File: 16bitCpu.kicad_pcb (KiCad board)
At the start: 4 copper layers, 73 parts, among them SW1 SW_Push, SW2 SW_SPDT, U1 74LS245, U10 74LS86, U11 74LS245, U12 74LS173, U13 74LS173, U14 74LS245, U15 74LS173, U16 74LS173, U17 74LS245, U18 74LS173, U19 74LS173, U2 74LS245, U20 74LS245, U21 74LS173, U22 74LS173, U23 LM555xN, U24 74LS04, U25 74LS08, U26 74LS32, U27 LM555xN, U28 LM555xN, U29 74LS245, U3 74LS283, U30 74LS245, U31 74LS161, U32 74LS161, U33 74LS161, U34 74LS161, U35 74HC00, U36 74LS245, U37 74HC04, U38 74LS173, U39 74LS173, U4 74LS283, U40 74LS245, U41 74LS173, U42 74LS173, U43 AS6C6264, U44 AS6C6264, U45 AT28C64B-15PU, U46 AT28C64B-15PU, U47 74LS245, U48 74LS173, U49 74LS173, U5 74LS283, U50 74LS245, U51 74LS173, U52 74LS173, U53 74LS173, U54 74HC02, U55 74HC02, U56 74LS08, U57 74LS08, U6 74LS283, U7 74LS86, U8 74LS86, U9 74LS86

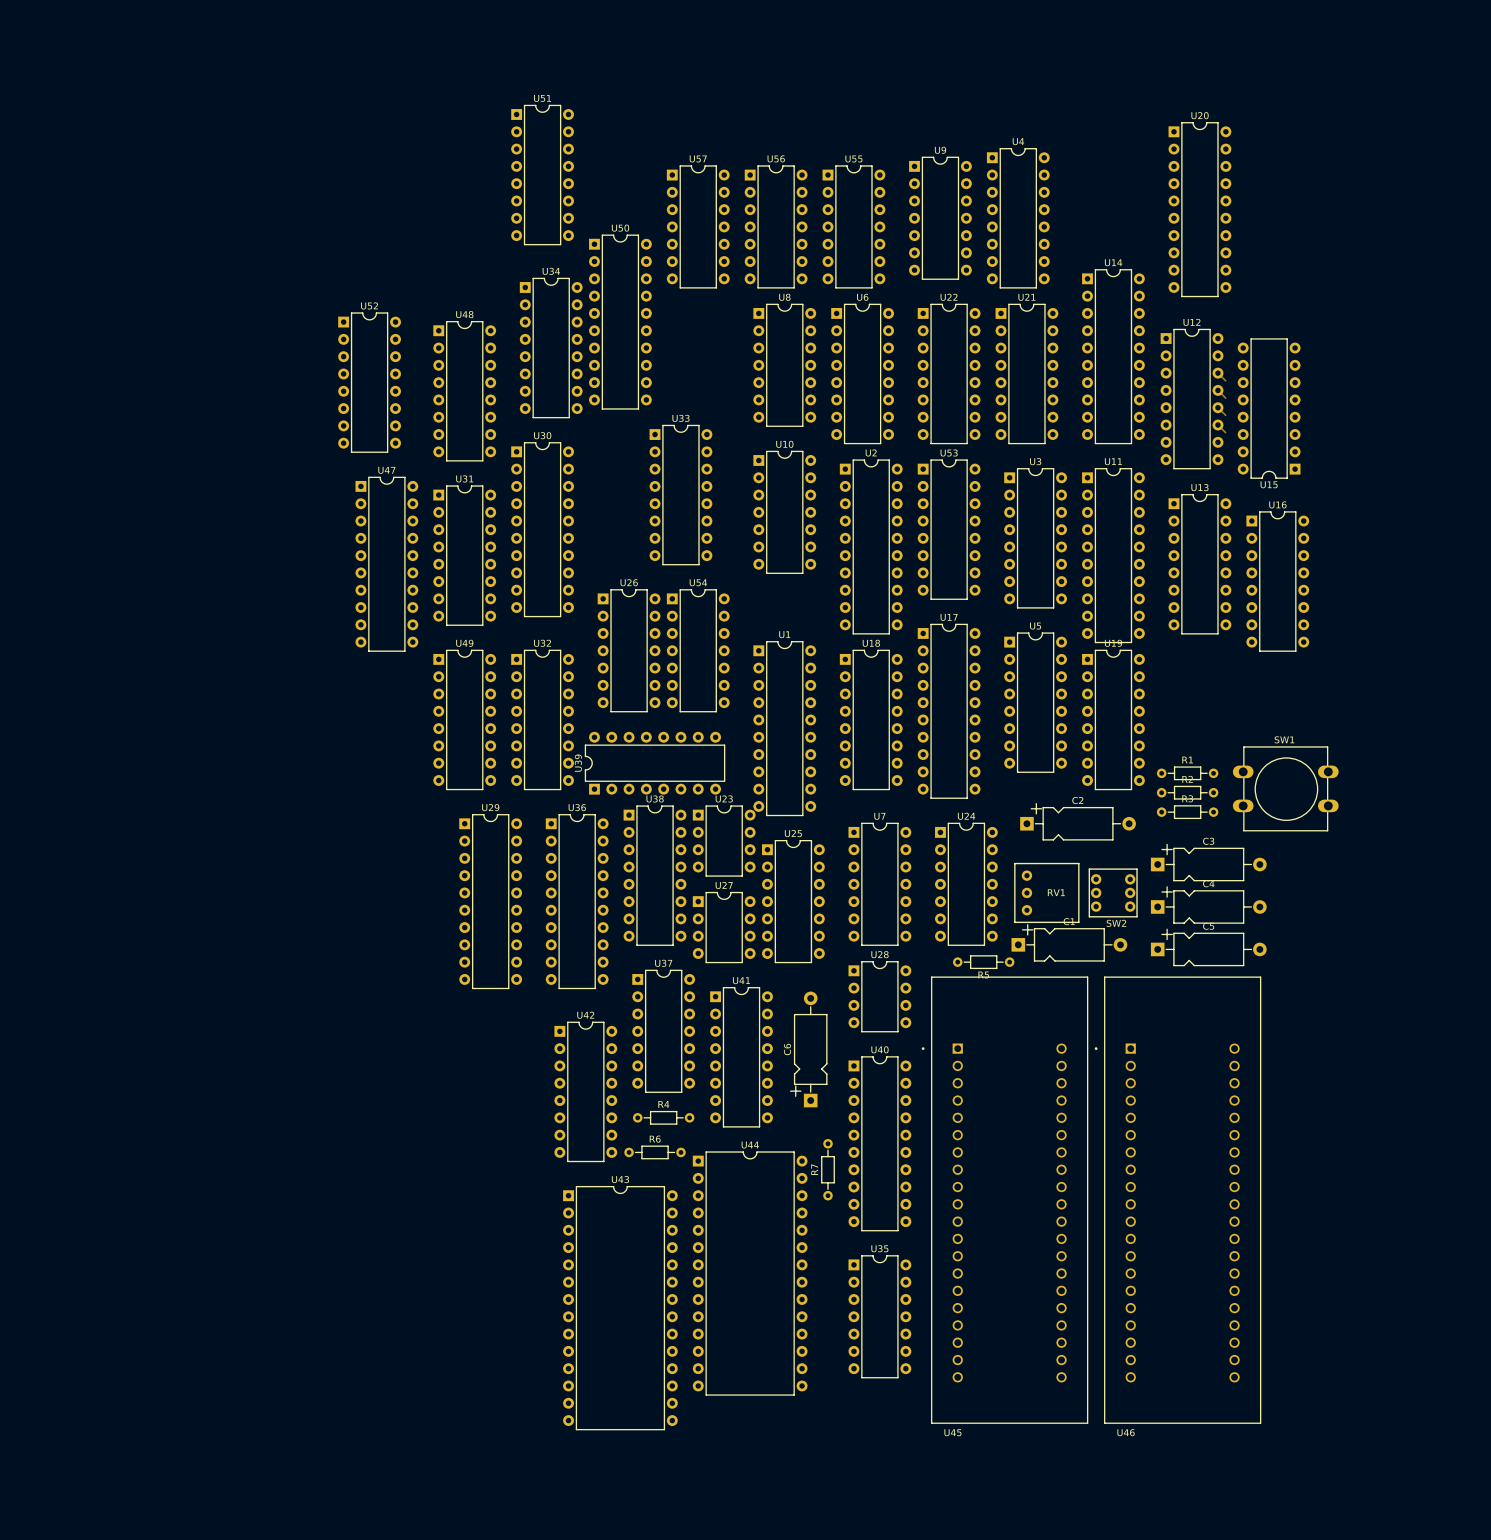
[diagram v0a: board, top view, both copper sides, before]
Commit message: made the CU , need to change the IR
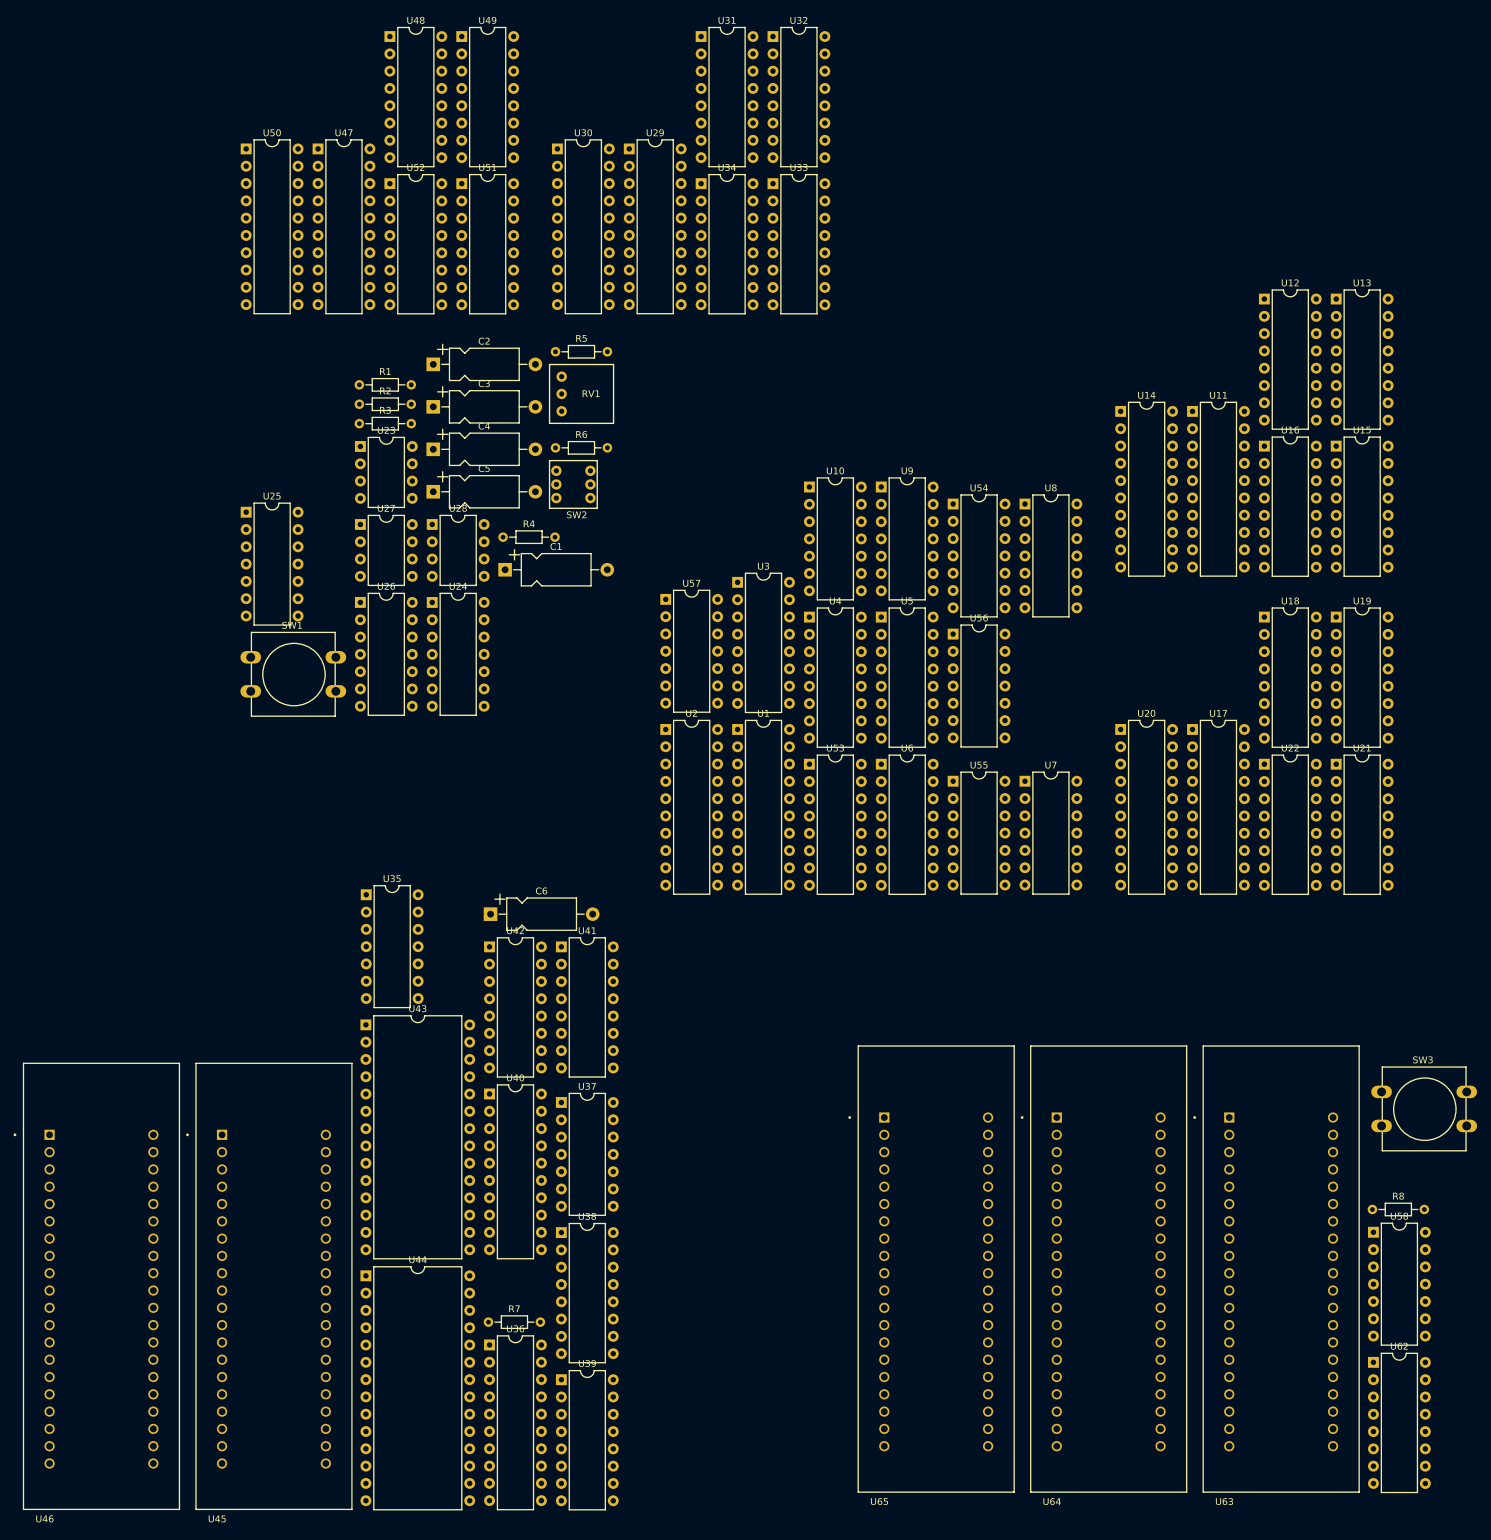
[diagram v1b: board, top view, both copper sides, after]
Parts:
- added R8: 1K, Resistor_THT:R_Axial_DIN0204_L3.6mm_D1.6mm_P7.62mm_Horizontal, F.Cu at (185.3, 209.0)
- added SW3: SW_Push-Switch, Button_Switch_THT:SW_PUSH-12mm, F.Cu at (186.7, 191.8)
- added U58: 7400, Package_DIP:DIP-14_W7.62mm, F.Cu at (185.5, 212.4)
- added U62: 74LS161-74xx, Package_DIP:DIP-16_W7.62mm, F.Cu at (185.5, 231.5)
- added U63: AT28C64B-15PU, ROM:ZIF-AT28C64B-15PU, F.Cu at (171.9, 219.7)
- added U64: AT28C64B-15PU, ROM:ZIF-AT28C64B-15PU, F.Cu at (146.6, 219.7)
- added U65: AT28C64B-15PU, ROM:ZIF-AT28C64B-15PU, F.Cu at (121.3, 219.7)
- moved U46 159.2 mm to (-1.26, 222.2)
- moved SW1 146.7 mm to (20.6, 128.0)
- moved R1 130.9 mm to (36.6, 88.0)
- moved R2 130.9 mm to (36.6, 90.8)
- moved R3 130.9 mm to (36.6, 93.7)
- moved C3 125.8 mm to (47.5, 91.2)
- moved C4 125.8 mm to (47.5, 97.4)
- moved C5 125.8 mm to (47.5, 103.7)
- moved R5 111.7 mm to (65.4, 83.1), turned to 0 degrees
- moved C2 110.2 mm to (47.5, 84.9)
- moved U45 108.8 mm to (24.1, 222.2)
- moved R6 104.0 mm to (65.4, 97.2)
- moved U29 102.0 mm to (76.2, 53.3)
- moved RV1 100.2 mm to (66.3, 91.8)
- moved SW2 99.4 mm to (65.5, 102.6)
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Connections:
- net /ALU/SU renamed /Control Unit/ALU_SU
- net /ALU/~EO renamed /Control Unit/~ALU_EO
- net /ALU/~FI renamed /Control Unit/~ALU_FI
- U53 pad 16: Net-(U53-Pad16) -> +5V
- U53 pad 8: Net-(U53-Pad8) -> GND
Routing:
- net /ALU/BUS0: track 1.59 -> 0.00 mm
- net /ALU/BUS3: track 1.59 -> 0.00 mm
- net /ALU/BUS2: track 1.59 -> 0.00 mm
- net /ALU/BUS1: track 1.59 -> 0.00 mm
